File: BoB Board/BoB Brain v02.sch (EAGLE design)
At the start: 43 parts, among them CN1 USB_CON, Q1 MOSFET-NCHANNELAO3404A, Q9 MOSFET-NCHANNELAO3404A, U1 ATMEGA328P_TQFP, U2 CH340G, U3 +12v, U4 V_REG_317SMD, Y1 16MHZ

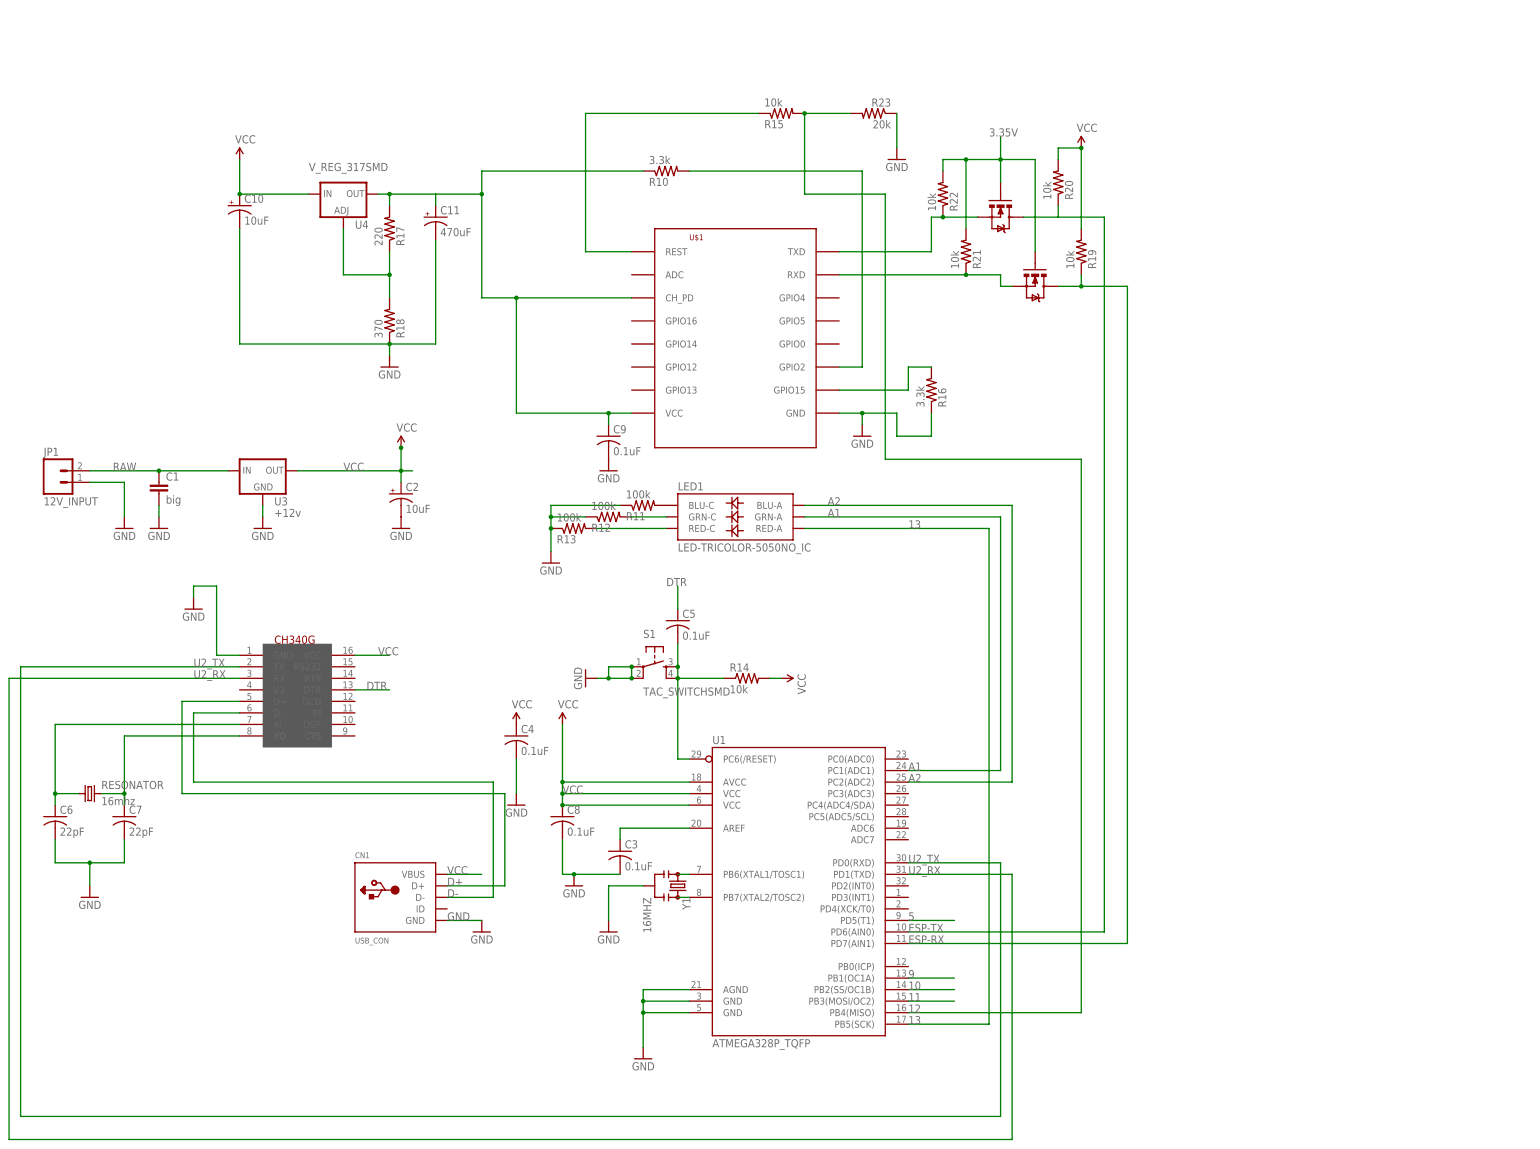
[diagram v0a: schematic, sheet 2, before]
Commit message: Working on BoB Board
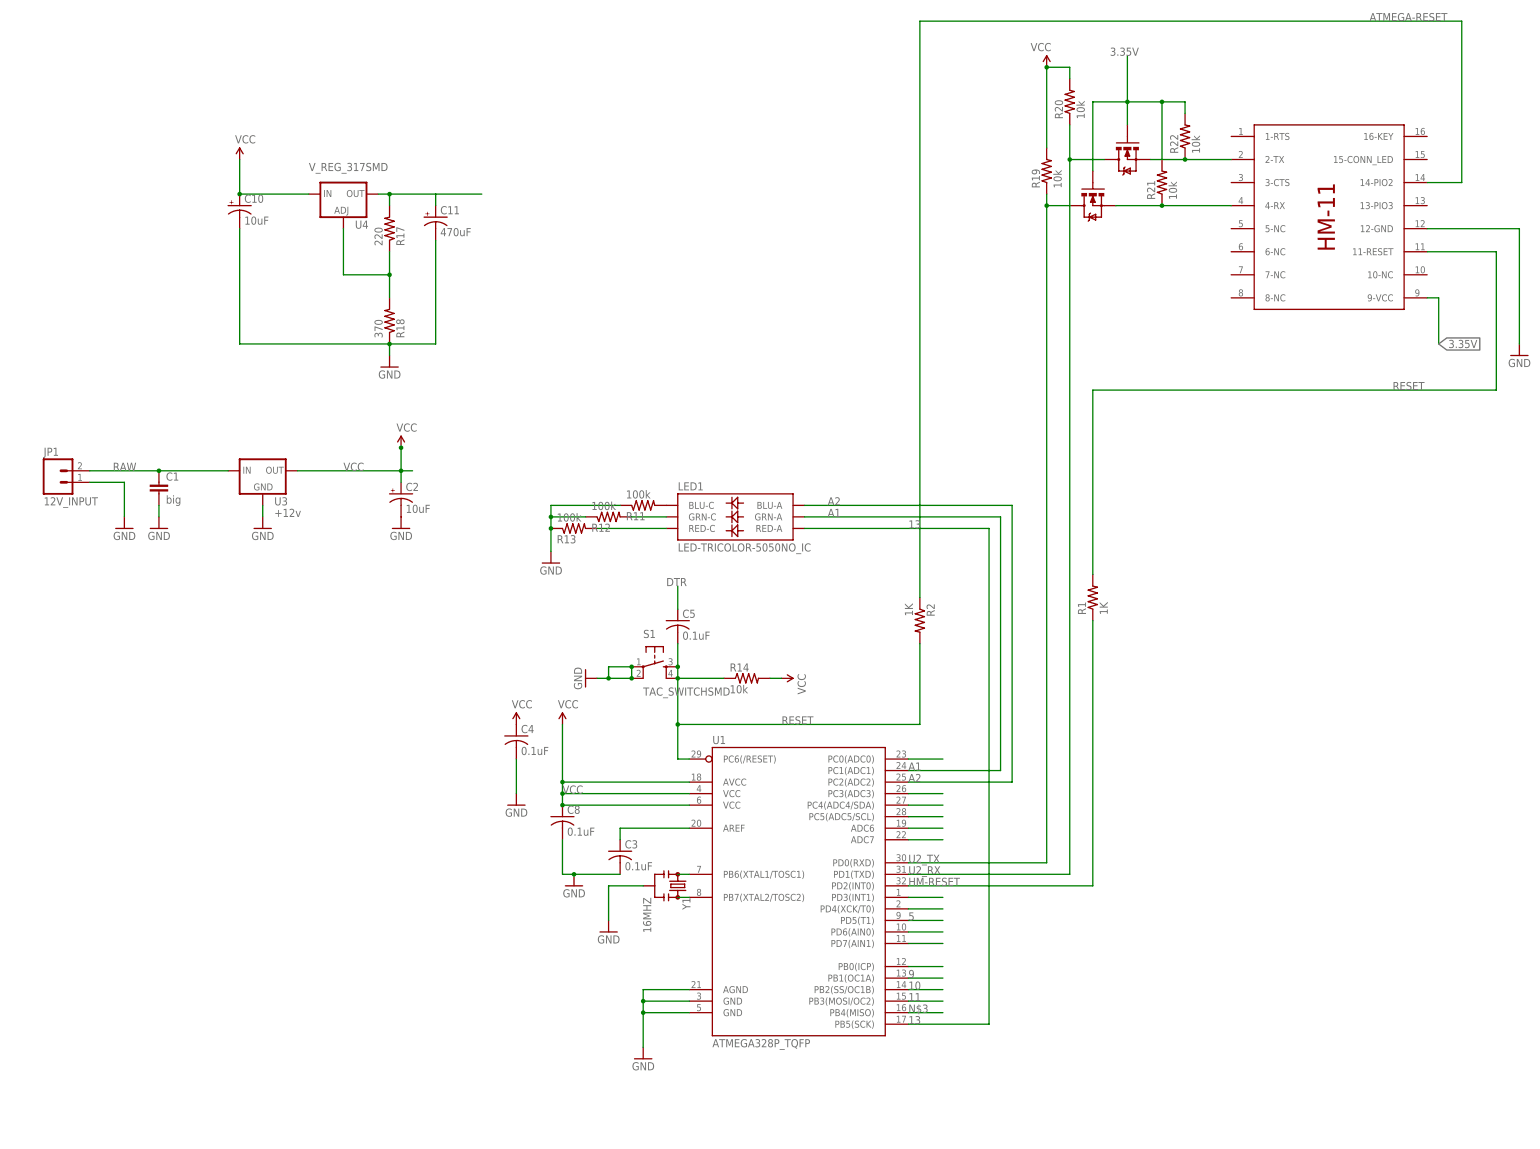
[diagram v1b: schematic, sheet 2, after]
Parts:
- removed C6, C7: 22pF, resistor:C-USC0805K
- removed C9: 0.1uF, resistor:C-USC0805K
- removed CN1: USB_CON, adafruit:USBMINIB
- removed R10, R16: 3.3k, resistor:R-US_R0805W
- removed R15: 10k, resistor:R-US_R0805W
- removed R23: 20k, resistor:R-US_R0805W
- removed RESONATOR: 16mhz, crystal:CRYSTALHC49UP
- removed U2: CH340G, usb-serial:CH340G
- added R1, R2: 1K, resistor:R-US_R0805W
- U$1: value ESP8266-07 -> HM-11; device lio:ESP8266-07 -> HM-11-ladvien:HM-11
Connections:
- removed net 12: R15.2, R23.2, U1.PB4(MISO)
- removed net D+: CN1.D+, U2.D+
- removed net D-: CN1.D-, U2.D-
- removed net ESP-RX: Q9.D, R19.1, U1.PD7(AIN1)
- removed net ESP-TX: Q1.D, R20.1, U1.PD6(AIN0)
- removed net X0: C7.1, RESONATOR.2, U2.XO
- removed net X1: C6.1, RESONATOR.1, U2.XI
- new net ATMEGA-RESET: R2.1, U$1.14-PIO2
- new net HM-RESET: R1.1, U1.PD2(INT0)
- new net N$26: U1.PC5(ADC5/SCL)
- new net N$27: U1.ADC6
- new net N$28: U1.ADC7
- new net N$29: U1.PD3(INT1)
- new net N$30: U1.PD4(XCK/T0)
- new net N$31: U1.PD6(AIN0)
- new net N$32: U1.PD7(AIN1)
- new net N$33: U1.PB0(ICP)
- new net RESET: C5.2, R1.2, R14.1, R2.2, S1.3, S1.4, U$1.11-RESET, U1.PC6(/RESET)
- net 3.35V: now also U$1.9-VCC; no longer C9.1, R10.1, U$1.CH_PD, U$1.VCC
- net DTR: no longer U2.DTR
- net GND: now also U$1.12-GND; no longer C6.2, C7.2, C9.2, CN1.GND, R16.1, R23.1, U$1.GND, U2.GND
- net N$12: now also U$1.2-TX; no longer U$1.TXD
- net N$13: now also U1.PC4(ADC4/SDA); no longer C5.2, R14.1, S1.3, S1.4, U1.PC6(/RESET)
- net N$15: now also U$1.4-RX; no longer U$1.RXD
- net N$3: now also U1.PB4(MISO); no longer R15.1, U$1.REST
- net N$4: now also U1.PC0(ADC0); no longer R10.2, U$1.GPIO2
- net N$5: now also U1.PC3(ADC3); no longer R16.2, U$1.GPIO15
- net U2_RX: now also Q1.D, R20.1; no longer U2.RX
- net U2_TX: now also Q9.D, R19.1; no longer U2.TX
- net VCC: no longer CN1.VBUS, U2.VCC
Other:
- moved on the sheet: R19, R20, R21, R22
